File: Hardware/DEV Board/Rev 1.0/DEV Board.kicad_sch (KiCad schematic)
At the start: 39 parts, among them J1 VBAT, J2 SPI, J3 PANEL, J4 6502 Card Connector, J5 6502 Bus, J6 USB Host, J7 USB HOST, J8 RJ45_LED, J9 ETHERNET, SW1 Run/Stop, SW2 Step, SW3 Clock, SW4 Reset, U1 SN74LVC4245APWR, U2 SN74LVC4245APWR, U3 SN74LVC4245APWR, U4 Teensy4.1, U5 SN74LVC4245APWR, U6 SN74LVC4245APWR

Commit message: Add BOMs
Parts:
- BT1: value BAT-HLD-001-THM -> CR2032; Availability In Stock -> (none); Check_prices https://www.snapeda.com/parts/BAT-HLD-001-THM/Linx+Technolo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 -> (none); Description_1 Holder for CR2032 and CR2025 Batteries, Through-Hole Mount,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 -> (none); Digikey (none) -> BAT-HLD-001-THM-ND; MF Linx Technologies -> (none); MP BAT-HLD-001-THM -> (none); Package None -> (none); Price None -> (none); Purchase-URL https://www.snapeda.com/api/url_track_click_mouser/?unipart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 -> (none); SnapEDA_Link https://www.snapeda.com/parts/BAT-HLD-001-THM/Linx+Technolo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 -> (none); now in the parts list
- J1, J2, J3, J7, J9: now in the parts list
- J4: Digikey (none) -> A31723-ND; now in the parts list
- J5: Other (none) -> https://www.amazon.com/Female-Headers-Connector-Header-Rasp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; now in the parts list
- J8: Digikey (none) -> 1278-1052-ND; now in the parts list
- U1, U2, U3, U5, U6: MF Texas Instruments -> (none); MP SN74LVC4245APWR -> (none); Package TSSOP-24 Texas Instruments -> (none)
- U4: Other (none) -> https://www.pjrc.com/store/teensy41.html; now in the parts list

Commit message: Finish BOM and add to README
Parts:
- BT1: Mouser (none) -> 712-BAT-HLD-001-THM
- J1, J7: Other (none) -> https://www.amazon.com/Straight-Breakaway-Connector-Breadbo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
- J2, J3: Other (none) -> https://www.amazon.com/Uxcell-Double-Straight-Header-Strip/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
- J4: Mouser (none) -> 571-5-5530843-4
- J9: Other (none) -> https://www.amazon.com/uxcell-2-0mm-Pitch-Double-Headers/dp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

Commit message: Restore exclude from BOM
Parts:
- BT1, J1, J2, J3, J4, J5, J7, J8, J9, U4: now left out of the parts list
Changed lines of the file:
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@@
 		(body_style 1)
 		(exclude_from_sim no)
-		(in_bom yes)
+		(in_bom no)
 		(on_board yes)
 		(in_pos_files yes)
@@
 		(body_style 1)
 		(exclude_from_sim no)
-		(in_bom yes)
+		(in_bom no)
 		(on_board yes)
 		(in_pos_files yes)
@@
 		(body_style 1)
 		(exclude_from_sim no)
-		(in_bom yes)
+		(in_bom no)
 		(on_board yes)
 		(in_pos_files yes)
@@
 		(body_style 1)
 		(exclude_from_sim no)
-		(in_bom yes)
+		(in_bom no)
 		(on_board yes)
 		(in_pos_files yes)
@@
 		(body_style 1)
 		(exclude_from_sim no)
-		(in_bom yes)
+		(in_bom no)
 		(on_board yes)
 		(in_pos_files no)
@@
 		(body_style 1)
 		(exclude_from_sim no)
-		(in_bom yes)
+		(in_bom no)
 		(on_board yes)
 		(in_pos_files yes)
@@
 		(body_style 1)
 		(exclude_from_sim no)
-		(in_bom yes)
+		(in_bom no)
 		(on_board yes)
 		(in_pos_files yes)
@@
 		(body_style 1)
 		(exclude_from_sim no)
-		(in_bom yes)
+		(in_bom no)
 		(on_board yes)
 		(in_pos_files yes)
@@
 		(body_style 1)
 		(exclude_from_sim no)
-		(in_bom yes)
+		(in_bom no)
 		(on_board yes)
 		(in_pos_files yes)
@@
 		(body_style 1)
 		(exclude_from_sim no)
-		(in_bom yes)
+		(in_bom no)
 		(on_board yes)
 		(in_pos_files yes)

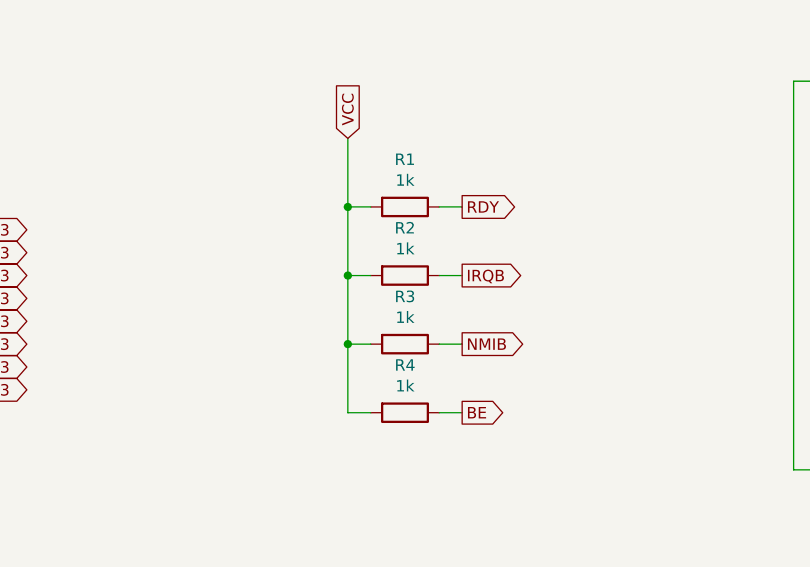
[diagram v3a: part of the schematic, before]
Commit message: Change pull up resistor values
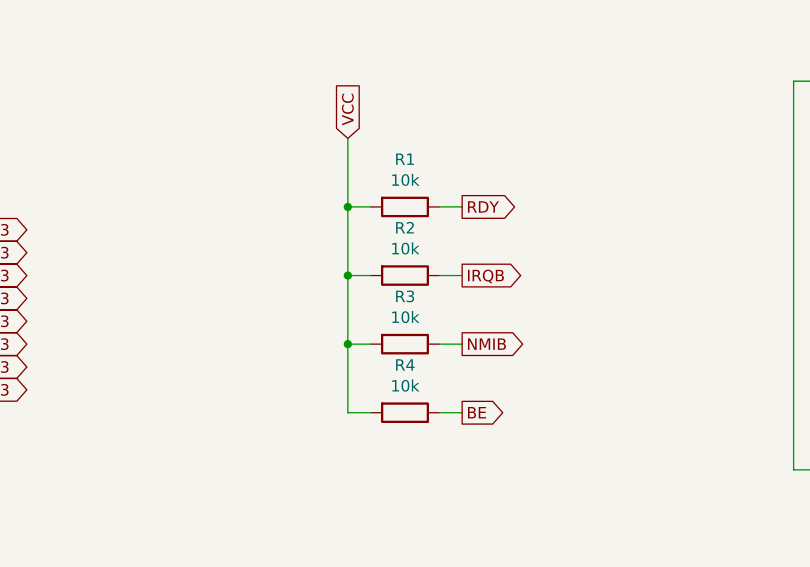
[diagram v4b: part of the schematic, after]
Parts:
- R1, R2, R3, R4: value 1k -> 10k; LCSC C17513 -> C2930231
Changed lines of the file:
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@@
 			)
 		)
-		(property "Value" "1k"
+		(property "Value" "10k"
 			(at 129.54 135.4836 90)
 			(show_name no)
@@
 			)
 		)
-		(property "LCSC" "C17513"
+		(property "LCSC" "C2930231"
 			(at 129.54 138.43 0)
 			(hide yes)
@@
 			)
 		)
-		(property "Value" "1k"
+		(property "Value" "10k"
 			(at 129.54 127.8636 90)
 			(show_name no)
@@
 			)
 		)
-		(property "LCSC" "C17513"
+		(property "LCSC" "C2930231"
 			(at 129.54 130.81 0)
 			(hide yes)
@@
 			)
 		)
-		(property "Value" "1k"
+		(property "Value" "10k"
 			(at 129.54 120.2436 90)
 			(show_name no)
@@
 			)
 		)
-		(property "LCSC" "C17513"
+		(property "LCSC" "C2930231"
 			(at 129.54 123.19 0)
 			(hide yes)
@@
 			)
 		)
-		(property "Value" "1k"
+		(property "Value" "10k"
 			(at 129.54 112.6236 90)
 			(show_name no)
@@
 			)
 		)
-		(property "LCSC" "C17513"
+		(property "LCSC" "C2930231"
 			(at 129.54 115.57 0)
 			(hide yes)

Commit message: Revert pull-up resistor value change
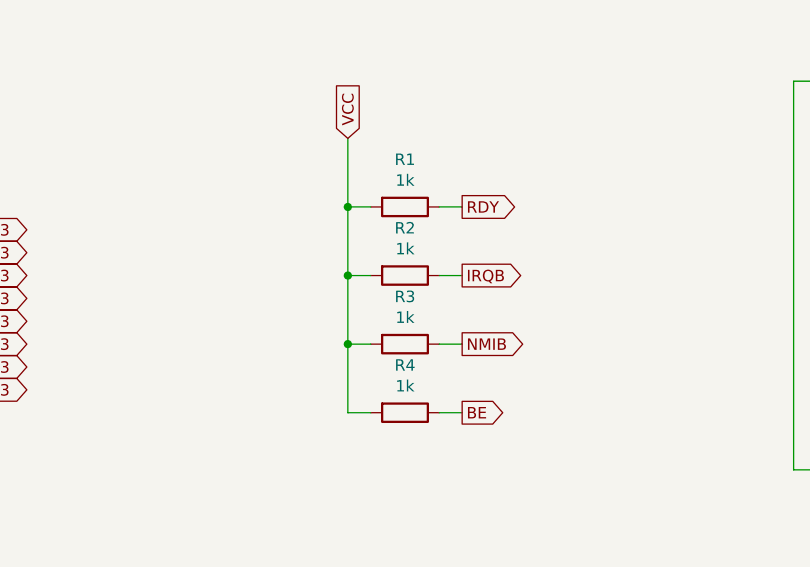
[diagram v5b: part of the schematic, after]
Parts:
- R1, R2, R3, R4: value 10k -> 1k; LCSC C2930231 -> C17513
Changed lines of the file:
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@@
 			)
 		)
-		(property "Value" "10k"
+		(property "Value" "1k"
 			(at 129.54 135.4836 90)
 			(show_name no)
@@
 			)
 		)
-		(property "LCSC" "C2930231"
+		(property "LCSC" "C17513"
 			(at 129.54 138.43 0)
 			(hide yes)
@@
 			)
 		)
-		(property "Value" "10k"
+		(property "Value" "1k"
 			(at 129.54 127.8636 90)
 			(show_name no)
@@
 			)
 		)
-		(property "LCSC" "C2930231"
+		(property "LCSC" "C17513"
 			(at 129.54 130.81 0)
 			(hide yes)
@@
 			)
 		)
-		(property "Value" "10k"
+		(property "Value" "1k"
 			(at 129.54 120.2436 90)
 			(show_name no)
@@
 			)
 		)
-		(property "LCSC" "C2930231"
+		(property "LCSC" "C17513"
 			(at 129.54 123.19 0)
 			(hide yes)
@@
 			)
 		)
-		(property "Value" "10k"
+		(property "Value" "1k"
 			(at 129.54 112.6236 90)
 			(show_name no)
@@
 			)
 		)
-		(property "LCSC" "C2930231"
+		(property "LCSC" "C17513"
 			(at 129.54 115.57 0)
 			(hide yes)
